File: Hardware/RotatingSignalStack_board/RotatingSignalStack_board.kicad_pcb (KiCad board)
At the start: 2 copper layers, 102 x 46.2 mm, 34 parts, among them J1 8P8C_LED_Shielded, SW1 SW_Push, SW2 SW_Push, U1 OKI, U2 Teensy4.1_DEV-16771

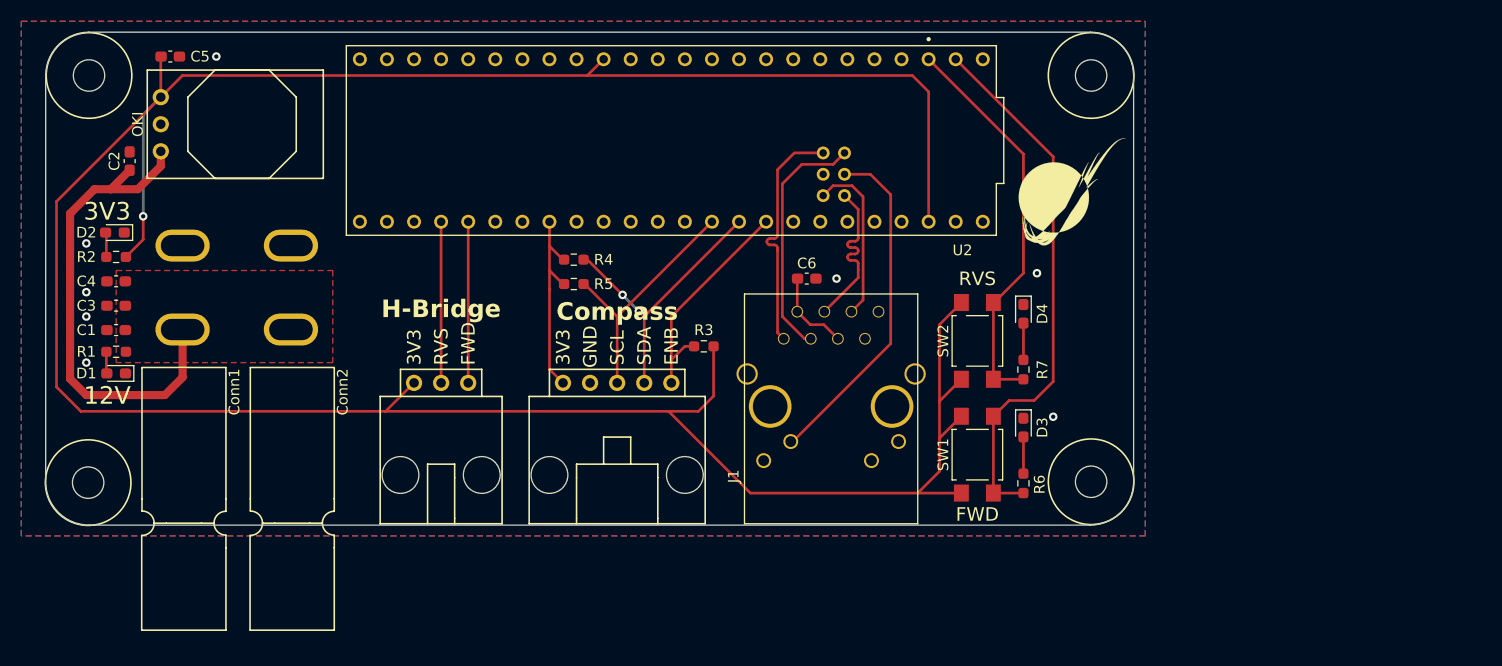
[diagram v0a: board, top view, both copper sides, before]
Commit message: Made Rev2 + Gerbs + STEP
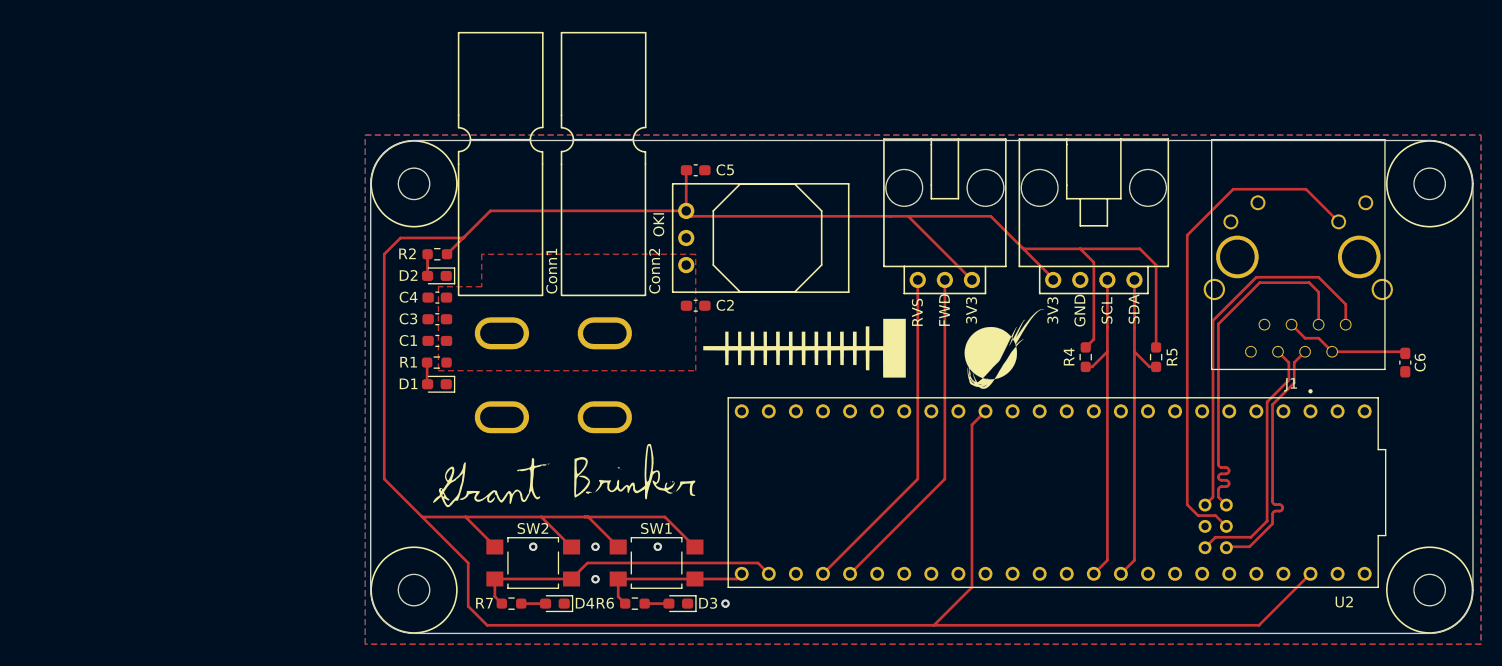
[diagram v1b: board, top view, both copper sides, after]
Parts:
- removed the G*** at (193.3, 82.0)
- removed the G*** at (128.3, 77.5)
- removed R3: 0, Resistor_SMD:R_0603_1608Metric_Pad0.98x0.95mm_HandSolder
- added G***: LOGO, MRDT_Silkscreens:0_MRDT_Logo_7.5mm, F.Cu at (186.9, 96.8)
- added G***: LOGO, MRDT_Silkscreens:0_MRDT_Logo_20mm, B.Cu at (164.8, 89.2)
- Conn3: value Molex_SL_05 -> Molex_SL_04; footprint MRDT_Connectors:MOLEX_SL_05_Horizontal -> MRDT_Connectors:MOLEX_SL_04_Horizontal
- G*** (x2): moved to F.Cu
- V1, V2, V3, V4: footprint MRDT_Drill_Holes:4_40_Hole_Corner -> MRDT_Drill_Holes:4_40_Hole
- moved V3 129.5 mm to (226.8, 119.4)
- moved V4 124.1 mm to (226.8, 81.3)
- moved V2 74.1 mm to (131.6, 119.4)
- moved V1 64.1 mm to (131.6, 81.3)
- moved J1 59.2 mm to (214.4, 75.1), turned to 180 degrees
- moved C6 56.7 mm to (224.5, 98.0), turned to -90 degrees
- moved R5 55.0 mm to (201.2, 97.5), turned to 90 degrees
- moved C2 54.8 mm to (158.0, 92.7), turned to 0 degrees
- moved R7 52.8 mm to (140.7, 120.7), turned to 0 degrees
- moved D4 51.7 mm to (144.8, 120.7), turned to 180 degrees
- moved C5 50.4 mm to (158.0, 80.0)
- moved U1 50.4 mm to (157.1, 88.9)
- moved R4 48.9 mm to (194.6, 97.5), turned to 90 degrees
- moved U2 48.7 mm to (191.5, 110.2)
- moved G*** 48.3 mm to (145.8, 108.7), turned to 0 degrees
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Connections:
- Conn3 pad 1: MAG ENABLE -> +3.3V
- Conn3 pad 2: I2C SDA -> GND
- Conn3 pad 4: GND -> I2C SDA
- Conn4 pad 1: HB_FWD -> HB_RVS
- Conn4 pad 2: HB_RVS -> HB_FWD
- R4 pad 1: COMP PWR -> I2C SCL
- R4 pad 2: I2C SDA -> +3.3V
- R5 pad 1: COMP PWR -> I2C SDA
- R5 pad 2: I2C SCL -> +3.3V
- U2 pad 0: JOG A -> unconnected-(U2-RX1-Pad0)
- U2 pad 1: JOG B -> unconnected-(U2-TX1-Pad1)
- U2 pad 18: MAG ENABLE -> unconnected-(U2-A4-Pad18)
- U2 pad 33: unconnected-(U2-MCLK2-Pad33) -> JOG A
- U2 pad 34: unconnected-(U2-RX8-Pad34) -> JOG B
- U2 pad 40: COMP PWR -> unconnected-(U2-A16-Pad40)
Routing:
- net +12V: track 46.1 -> 0.00 mm
- net JOG A: track 51.0 -> 14.4 mm
- net +3.3V: track 266.8 -> 291.9 mm, vias 1 -> 0
- net MAG ENABLE: track 21.5 -> 0.00 mm
- net COMP PWR: track 19.4 -> 0.00 mm
- net HB_RVS: track 15.1 -> 31.2 mm
- net HB_FWD: track 15.1 -> 31.2 mm
- net /LED: track 32.3 -> 47.0 mm
- net /Tx+: track 22.5 -> 34.7 mm
- net /Tx-: track 23.0 -> 34.6 mm
- net JOG B: track 37.7 -> 29.3 mm
- net /Rx+: track 15.6 -> 24.0 mm
- net /Rx-: track 15.8 -> 24.0 mm
- net I2C SCL: track 23.2 -> 30.7 mm
- net I2C SDA: track 26.7 -> 30.7 mm, vias 2 -> 0
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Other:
- board size 102 x 46.2 mm -> 103.4 x 46.2 mm
- board text added: "Signal Stack Board, Rev2 Mars Rover Design Team Missouri S&T, 2024 Grant Brinker"
- board text removed: "12V"
- board text removed: "Compass"
- board text removed: "ENB"
- board text removed: "H-Bridge"
- board text removed: "Signal Stack Board, Rev1 Mars Rover Design Team Missouri S&T, 2024 Grant Brinker"
